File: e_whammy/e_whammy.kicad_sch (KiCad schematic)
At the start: 16 parts, among them J1 I/O connector, U1 HT7550-1, U2 DRV5056, U3 TLV6001UIDBVR

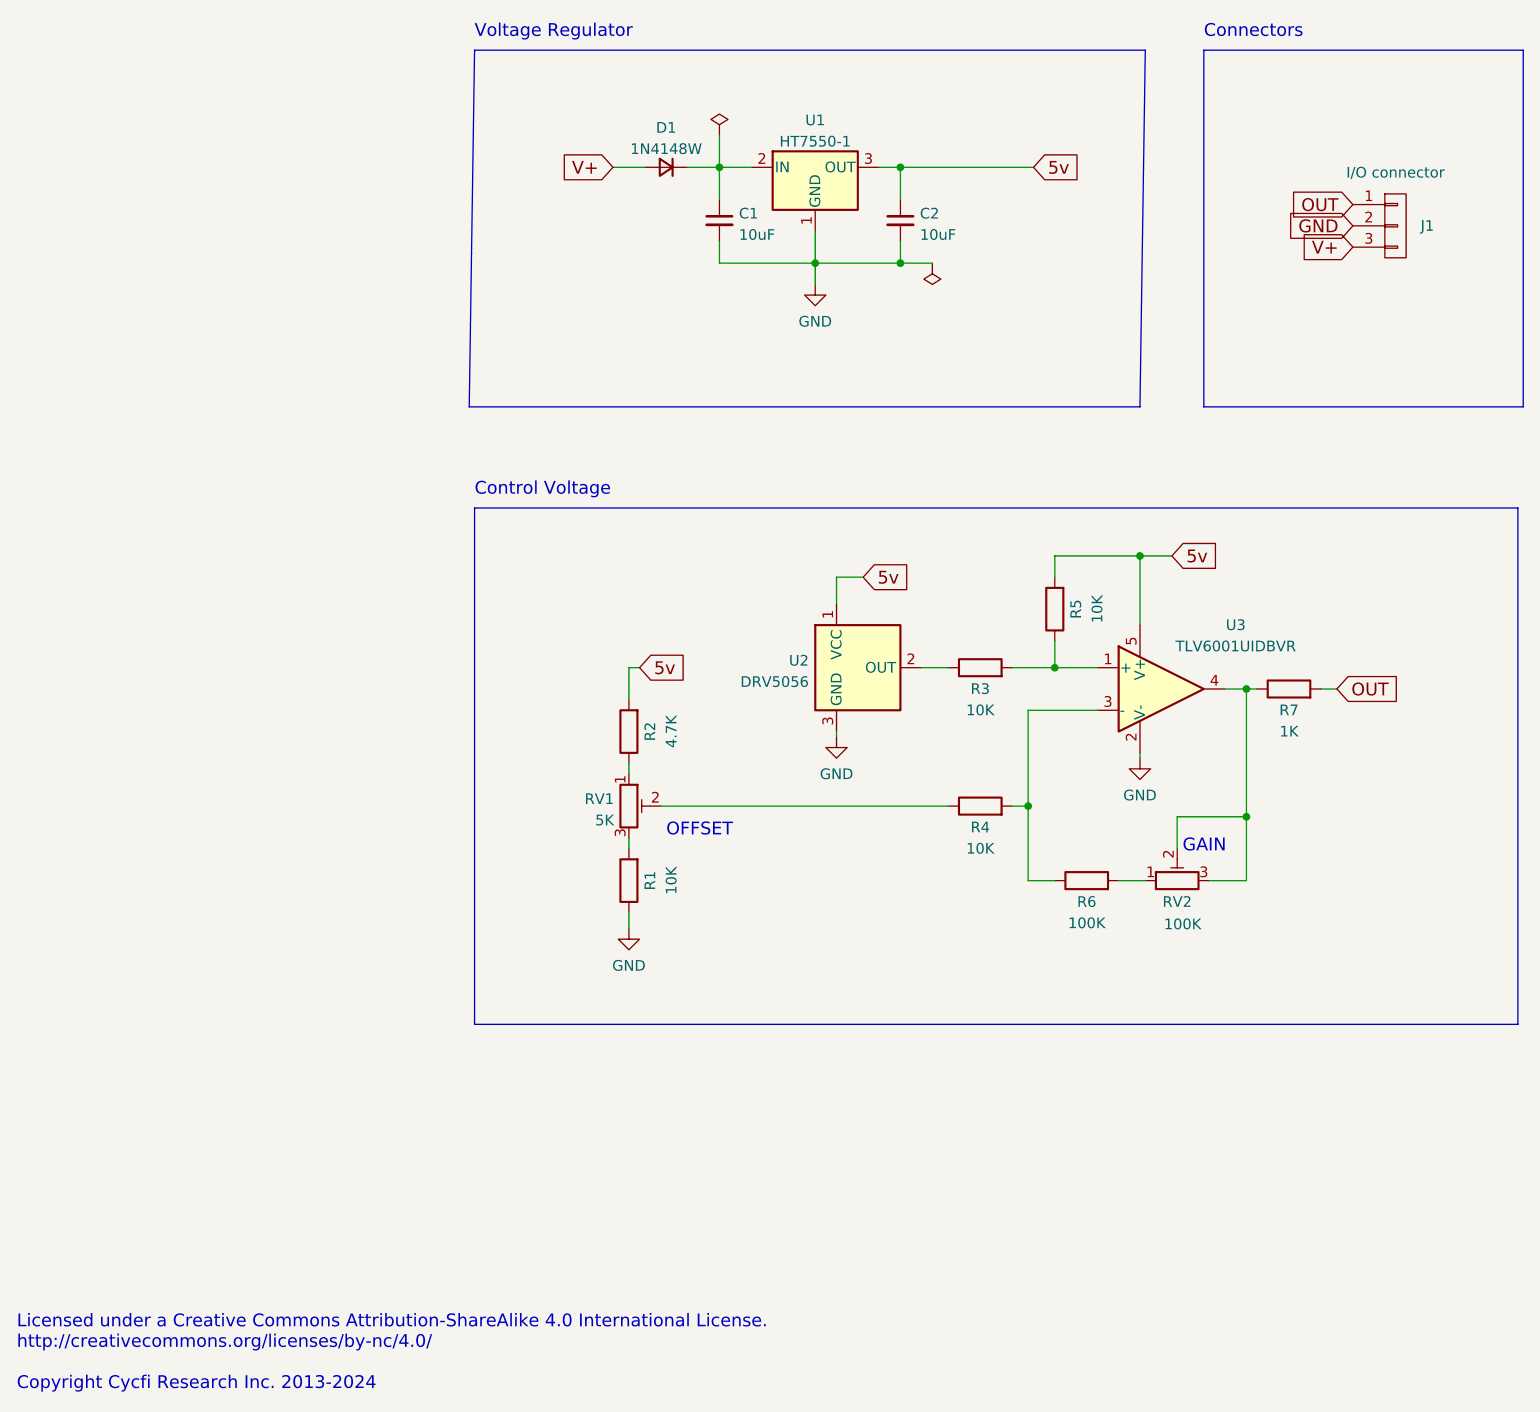
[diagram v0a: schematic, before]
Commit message: New uni-mount version
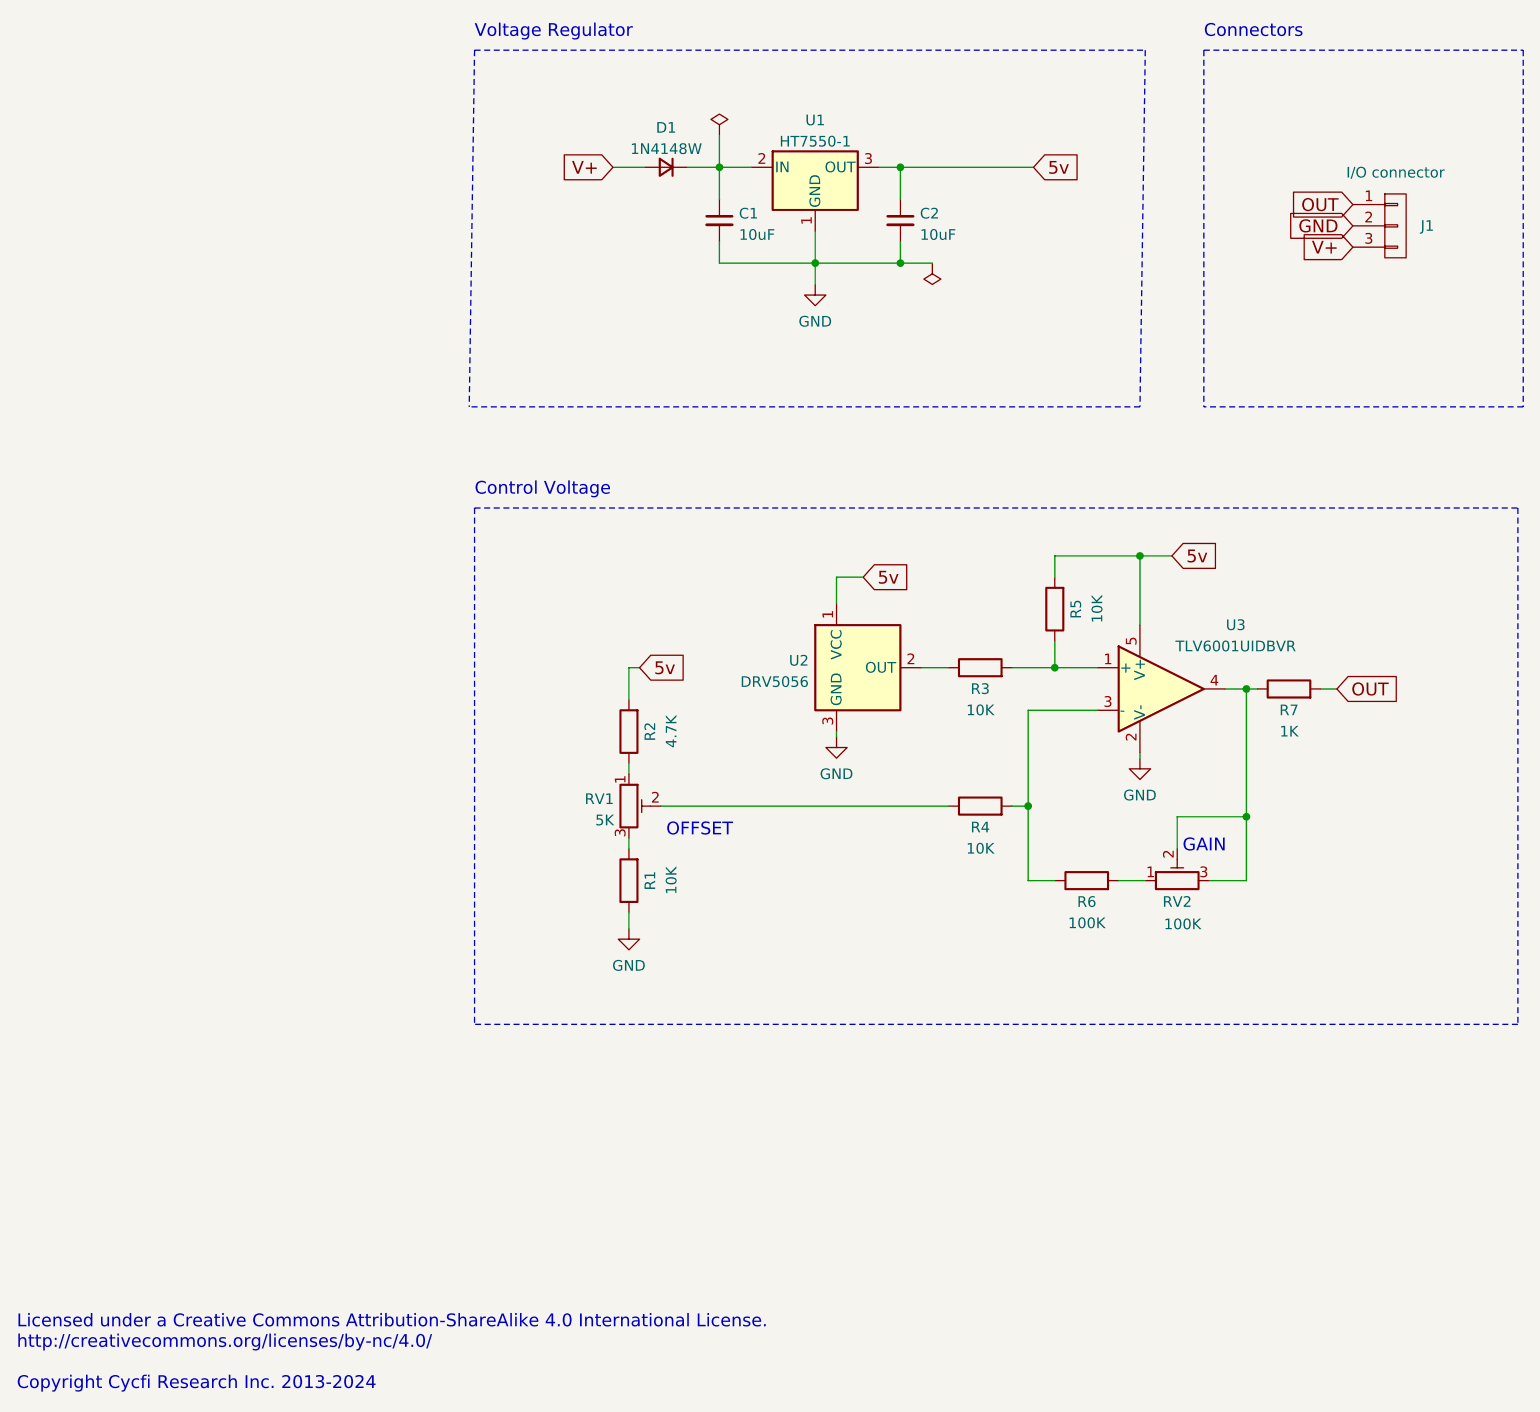
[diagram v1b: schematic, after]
